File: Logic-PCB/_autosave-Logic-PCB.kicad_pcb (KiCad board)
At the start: 2 copper layers, 148 parts, among them IC1 74LVC1G74DC-Q100H, IC10 SN74LVC1G11MDCKREP, IC11 SN74LVC1G11MDCKREP, IC12 74AUP1G32GW-Q100H, IC13 TMUX1208QRSVRQ1, IC14 TMUX1208QRSVRQ1, IC15 TMUX1208QRSVRQ1, IC16 TMUX1208QRSVRQ1, IC17 TMUX1208QRSVRQ1, IC18 TMUX1208QRSVRQ1, IC19 TMUX1208QRSVRQ1, IC2 74HC73D,653, IC20 TMUX1208QRSVRQ1, IC21 TMUX1208QRSVRQ1, IC3 SN74LVC1G02DBVR, IC4 SN74LVC1G02DBVR, IC5 74AUP1T87GWH, IC6 NCV4274CDT33RKG, IC7 74HC73D,653, IC8 TLC555QDRQ1, IC9 74HC73D,653, J1 CX70M-24P1, Q1 BC847,215, Q10 PMV100EPAR, Q11 2N7002_HAMR, Q12 2N7002_HAMR, Q13 BC858B,235, Q2 BC847,215, Q3 BC847,215, Q4 BC847,215, Q5 PMV100EPAR, Q6 PMV100EPAR, Q7 2N7002_HAMR, Q8 2N7002_HAMR, Q9 PMV100EPAR, SW1 SW_Push, SW2 SW_Push, U1 74AHC1G86W5-7, U3 NC7S08M5X

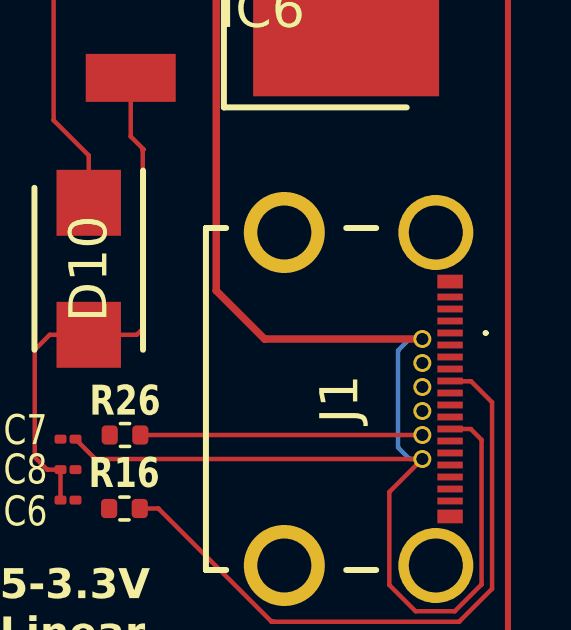
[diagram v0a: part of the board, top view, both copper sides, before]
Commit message: Routing and LEDs
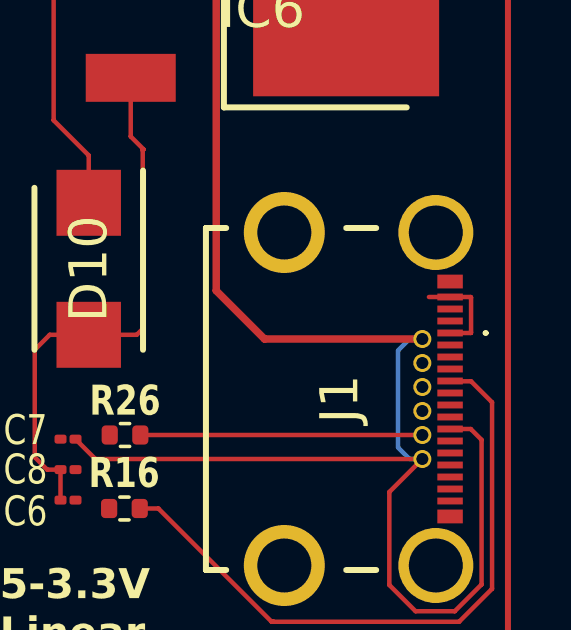
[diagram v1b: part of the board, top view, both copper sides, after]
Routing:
- net GND: track 27.0 -> 30.3 mm
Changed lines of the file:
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@@
   (segment (start 104.94 45.49) (end 105.34 45.89) (width 0.15) (layer "F.Cu") (net 131))
   (segment (start 113.24 50.85) (end 113.24 50.144974) (width 0.15) (layer "F.Cu") (net 131))
+  (segment (start 142.535 79.275) (end 142.52 79.26) (width 0.15) (layer "F.Cu") (net 131))
   (segment (start 106.14 37.91) (end 106.14 38.35) (width 0.15) (layer "F.Cu") (net 131))
   (segment (start 106.14 53.02) (end 106.14 53.57) (width 0.15) (layer "F.Cu") (net 131))
@@
   (segment (start 113.64 50.85) (end 113.24 50.85) (width 0.15) (layer "F.Cu") (net 131))
   (segment (start 112.84 40.82) (end 112.84 40.27) (width 0.15) (layer "F.Cu") (net 131))
+  (segment (start 142.535 80.45) (end 142.535 79.275) (width 0.15) (layer "F.Cu") (net 131))
   (segment (start 106.74 45.54) (end 106.74 45.14) (width 0.15) (layer "F.Cu") (net 131))
   (segment (start 106.14 52.62) (end 106.19 52.57) (width 0.15) (layer "F.Cu") (net 131))
   (segment (start 112.84 49.744974) (end 112.84 49.25) (width 0.15) (layer "F.Cu") (net 131))
   (segment (start 104.94 38.46) (end 105.34 38.86) (width 0.15) (layer "F.Cu") (net 131))
+  (segment (start 141.835 80.46) (end 142.525 80.46) (width 0.15) (layer "F.Cu") (net 131))
   (segment (start 114.64 40.87) (end 112.89 40.87) (width 0.15) (layer "F.Cu") (net 131))
   (segment (start 120.83 67.58) (end 121.36 68.11) (width 0.15) (layer "F.Cu") (net 131))
@@
   (segment (start 113.24 41.87) (end 114.04 41.87) (width 0.15) (layer "F.Cu") (net 131))
   (segment (start 114.64 41.67) (end 114.64 41.79) (width 0.15) (layer "F.Cu") (net 131))
+  (segment (start 141.835 79.26) (end 141.13 79.26) (width 0.15) (layer "F.Cu") (net 131))
   (segment (start 106.19 52.57) (end 106.74 52.57) (width 0.15) (layer "F.Cu") (net 131))
   (segment (start 114.56 41.87) (end 114.04 41.87) (width 0.15) (layer "F.Cu") (net 131))
   (segment (start 106.74 52.17) (end 106.74 52.57) (width 0.15) (layer "F.Cu") (net 131))
+  (segment (start 142.52 79.26) (end 141.835 79.26) (width 0.15) (layer "F.Cu") (net 131))
   (segment (start 106.14 53.02) (end 106.14 52.62) (width 0.15) (layer "F.Cu") (net 131))
   (segment (start 106.74 53.46) (end 106.63 53.57) (width 0.15) (layer "F.Cu") (net 131))
@@
   (segment (start 121.66 69.89) (end 122.165 69.89) (width 0.15) (layer "F.Cu") (net 131))
   (segment (start 113.64 49.25) (end 114.04 49.25) (width 0.15) (layer "F.Cu") (net 131))
+  (segment (start 142.525 80.46) (end 142.535 80.45) (width 0.15) (layer "F.Cu") (net 131))
   (segment (start 106.14 51.97) (end 106.14 53.57) (width 0.15) (layer "F.Cu") (net 131))
   (segment (start 106.14 39.51) (end 106.14 38.35) (width 0.15) (layer "F.Cu") (net 131))
